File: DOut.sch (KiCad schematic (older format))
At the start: 2 parts, among them J24 Conn_02x10_Odd_Even

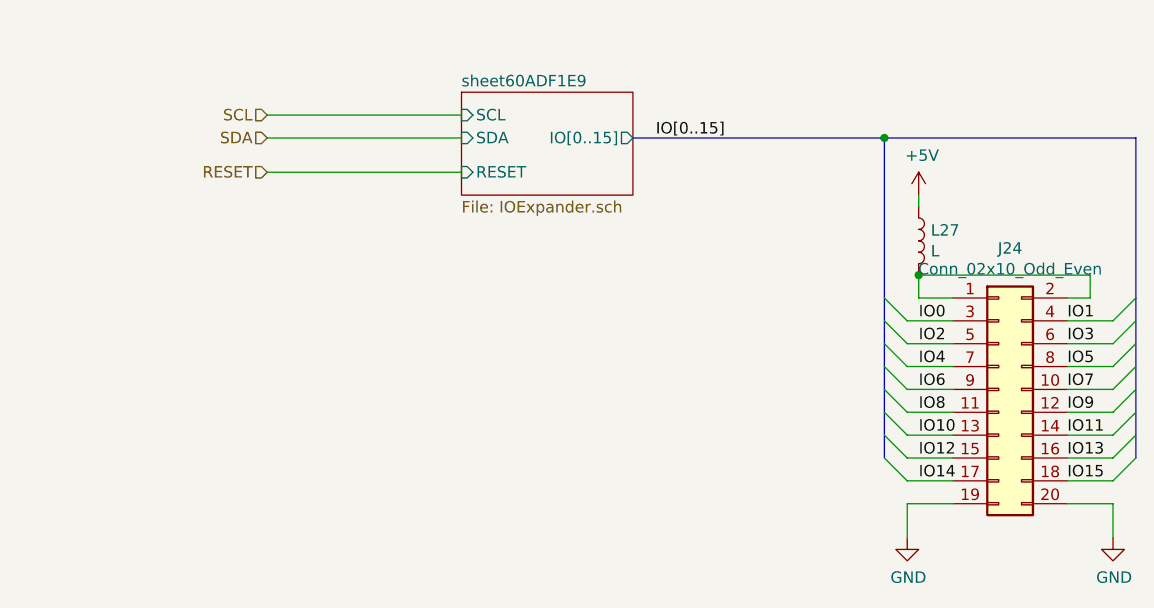
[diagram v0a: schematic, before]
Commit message: ready for jlc
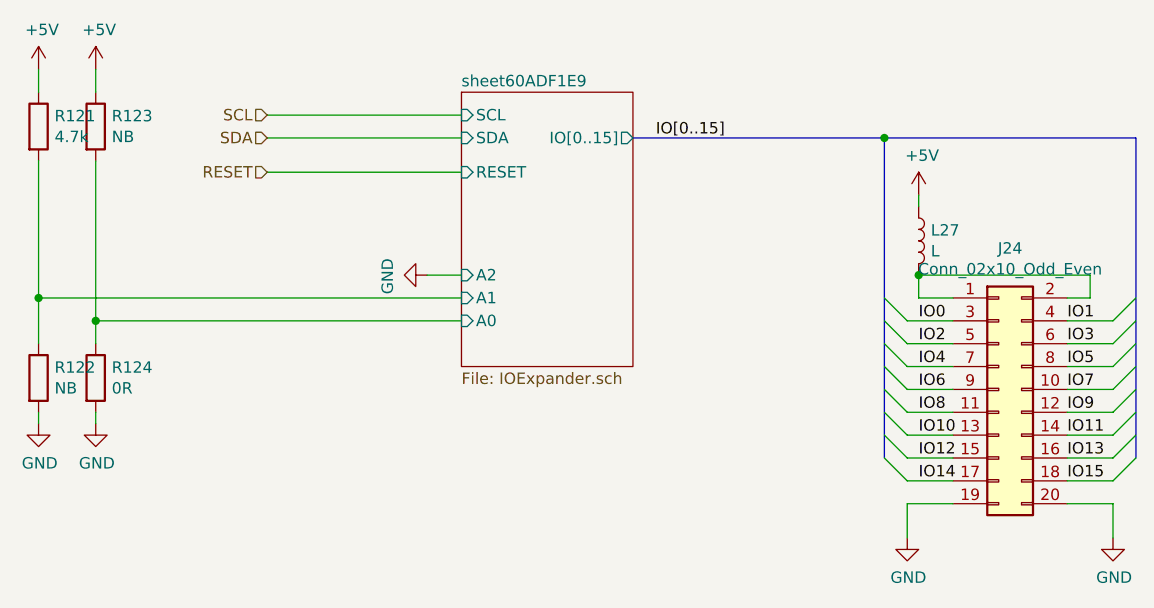
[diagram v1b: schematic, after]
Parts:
- added R121: 4.7k, Resistor_SMD:R_0603_1608Metric, symbol AR2ISS:R
- added R122, R123: NB, Resistor_SMD:R_0603_1608Metric, symbol AR2ISS:R
- added R124: 0R, Resistor_SMD:R_0603_1608Metric, symbol AR2ISS:R
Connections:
- net +5V: now also R121.1, R123.1
- net GND: now also R122.2, R124.2
- new net sheet60ADF1E9/A0: R123.2, R124.1
- new net sheet60ADF1E9/A1: R121.2, R122.1
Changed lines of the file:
@@
 $Descr A4 11693 8268
 encoding utf-8
-Sheet 12 22
+Sheet 11 22
 Title ""
 Date ""
@@
 $EndDescr
 $Sheet
-S 4650 2300 750  450
+S 4650 2300 750  1200
 U 60ADF1EF
 F0 "sheet60ADF1E9" 50
@@
 F4 "RESET" I L 4650 2650 50
 F5 "IO[0..15]" O R 5400 2500 50
+F6 "A0" I L 4650 3300 50
+F7 "A1" I L 4650 3200 50
+F8 "A2" I L 4650 3100 50
 $EndSheet
 Text HLabel 3800 2400 0    50   Input ~ 0
@@
 Text Label 7300 4000 0    50   ~ 0
 IO15
+$Comp
+L AR2ISS:R R?
+U 1 1 60A7591A
+P 3050 3550
+AR Path="/60679D69/60A7591A" Ref="R?"  Part="1"
+AR Path="/607267A8/60A7591A" Ref="R?"  Part="1"
+AR Path="/60A2B663/60A7591A" Ref="R?"  Part="1"
+AR Path="/60A2BC9C/60A7591A" Ref="R?"  Part="1"
+AR Path="/60ADDFFD/60A7591A" Ref="R?"  Part="1"
+AR Path="/60ADEB0F/60ADF1EF/60A7591A" Ref="R?"  Part="1"
+AR Path="/60A7591A" Ref="R?"  Part="1"
+AR Path="/60ADEB0F/60A7591A" Ref="R124"  Part="1"
+F 0 "R124" H 3120 3596 50  0000 L CNN
+F 1 "0R" H 3120 3505 50  0000 L CNN
+F 2 "Resistor_SMD:R_0603_1608Metric" V 2980 3550 50  0001 C CNN
+F 3 "~" H 3050 3550 50  0001 C CNN
+	1    3050 3550
+	1    0    0    -1
+$EndComp
+$Comp
+L power:GND #PWR?
+U 1 1 60A75920
+P 3050 3750
+AR Path="/607267A8/60A75920" Ref="#PWR?"  Part="1"
+AR Path="/60679D69/60A75920" Ref="#PWR?"  Part="1"
+AR Path="/60A2B663/60A75920" Ref="#PWR?"  Part="1"
+AR Path="/60A2BC9C/60A75920" Ref="#PWR?"  Part="1"
+AR Path="/60ADDFFD/60A75920" Ref="#PWR?"  Part="1"
+AR Path="/60ADEB0F/60ADF1EF/60A75920" Ref="#PWR?"  Part="1"
+AR Path="/60A75920" Ref="#PWR?"  Part="1"
+AR Path="/60ADEB0F/60A75920" Ref="#PWR0176"  Part="1"
+F 0 "#PWR0176" H 3050 3500 50  0001 C CNN
+F 1 "GND" H 3055 3577 50  0000 C CNN
+F 2 "" H 3050 3750 50  0001 C CNN
+F 3 "" H 3050 3750 50  0001 C CNN
+	1    3050 3750
+	1    0    0    -1
+$EndComp
+Wire Wire Line
+	3050 3700 3050 3750
+$Comp
+L AR2ISS:R R?
+U 1 1 60A75927
+P 2800 3550
+AR Path="/60679D69/60A75927" Ref="R?"  Part="1"
+AR Path="/607267A8/60A75927" Ref="R?"  Part="1"
+AR Path="/60A2B663/60A75927" Ref="R?"  Part="1"
+AR Path="/60A2BC9C/60A75927" Ref="R?"  Part="1"
+AR Path="/60ADDFFD/60A75927" Ref="R?"  Part="1"
+AR Path="/60ADEB0F/60ADF1EF/60A75927" Ref="R?"  Part="1"
+AR Path="/60A75927" Ref="R?"  Part="1"
+AR Path="/60ADEB0F/60A75927" Ref="R122"  Part="1"
+F 0 "R122" H 2870 3596 50  0000 L CNN
+F 1 "NB" H 2870 3505 50  0000 L CNN
+F 2 "Resistor_SMD:R_0603_1608Metric" V 2730 3550 50  0001 C CNN
+F 3 "~" H 2800 3550 50  0001 C CNN
+	1    2800 3550
+	1    0    0    -1
+$EndComp
+$Comp
+L power:GND #PWR?
+U 1 1 60A7592D
+P 2800 3750
+AR Path="/607267A8/60A7592D" Ref="#PWR?"  Part="1"
+AR Path="/60679D69/60A7592D" Ref="#PWR?"  Part="1"
+AR Path="/60A2B663/60A7592D" Ref="#PWR?"  Part="1"
+AR Path="/60A2BC9C/60A7592D" Ref="#PWR?"  Part="1"
+AR Path="/60ADDFFD/60A7592D" Ref="#PWR?"  Part="1"
+AR Path="/60ADEB0F/60ADF1EF/60A7592D" Ref="#PWR?"  Part="1"
+AR Path="/60A7592D" Ref="#PWR?"  Part="1"
+AR Path="/60ADEB0F/60A7592D" Ref="#PWR0177"  Part="1"
+F 0 "#PWR0177" H 2800 3500 50  0001 C CNN
+F 1 "GND" H 2805 3577 50  0000 C CNN
+F 2 "" H 2800 3750 50  0001 C CNN
+F 3 "" H 2800 3750 50  0001 C CNN
+	1    2800 3750
+	1    0    0    -1
+$EndComp
+Wire Wire Line
+	2800 3700 2800 3750
+$Comp
+L power:+5V #PWR?
+U 1 1 60A75934
+P 3050 2200
+AR Path="/607267A8/60A75934" Ref="#PWR?"  Part="1"
+AR Path="/60679D69/60A75934" Ref="#PWR?"  Part="1"
+AR Path="/60A2B663/60A75934" Ref="#PWR?"  Part="1"
+AR Path="/60A2BC9C/60A75934" Ref="#PWR?"  Part="1"
+AR Path="/60ADDFFD/60A75934" Ref="#PWR?"  Part="1"
+AR Path="/60ADEB0F/60ADF1EF/60A75934" Ref="#PWR?"  Part="1"
+AR Path="/60A75934" Ref="#PWR?"  Part="1"
+AR Path="/60ADEB0F/60A75934" Ref="#PWR0178"  Part="1"
+F 0 "#PWR0178" H 3050 2050 50  0001 C CNN
+F 1 "+5V" H 3065 2373 50  0000 C CNN
+F 2 "" H 3050 2200 50  0001 C CNN
+F 3 "" H 3050 2200 50  0001 C CNN
+	1    3050 2200
+	1    0    0    -1
+$EndComp
+$Comp
+L power:+5V #PWR?
+U 1 1 60A7593A
+P 2800 2200
+AR Path="/607267A8/60A7593A" Ref="#PWR?"  Part="1"
+AR Path="/60679D69/60A7593A" Ref="#PWR?"  Part="1"
+AR Path="/60A2B663/60A7593A" Ref="#PWR?"  Part="1"
+AR Path="/60A2BC9C/60A7593A" Ref="#PWR?"  Part="1"
+AR Path="/60ADDFFD/60A7593A" Ref="#PWR?"  Part="1"
+AR Path="/60ADEB0F/60ADF1EF/60A7593A" Ref="#PWR?"  Part="1"
+AR Path="/60A7593A" Ref="#PWR?"  Part="1"
+AR Path="/60ADEB0F/60A7593A" Ref="#PWR0213"  Part="1"
+F 0 "#PWR0213" H 2800 2050 50  0001 C CNN
+F 1 "+5V" H 2815 2373 50  0000 C CNN
+F 2 "" H 2800 2200 50  0001 C CNN
+F 3 "" H 2800 2200 50  0001 C CNN
+	1    2800 2200
+	1    0    0    -1
+$EndComp
+Wire Wire Line
+	2800 3200 2800 3400
+Connection ~ 2800 3200
+Wire Wire Line
+	3050 3400 3050 3300
+Connection ~ 3050 3300
+Wire Wire Line
+	2800 3200 4650 3200
+Wire Wire Line
+	3050 3300 4650 3300
+$Comp
+L AR2ISS:R R?
+U 1 1 60A75947
+P 2800 2450
+AR Path="/60679D69/60A75947" Ref="R?"  Part="1"
+AR Path="/607267A8/60A75947" Ref="R?"  Part="1"
+AR Path="/60A2B663/60A75947" Ref="R?"  Part="1"
+AR Path="/60A2BC9C/60A75947" Ref="R?"  Part="1"
+AR Path="/60ADDFFD/60A75947" Ref="R?"  Part="1"
+AR Path="/60ADEB0F/60ADF1EF/60A75947" Ref="R?"  Part="1"
+AR Path="/60A75947" Ref="R?"  Part="1"
+AR Path="/60ADEB0F/60A75947" Ref="R121"  Part="1"
+F 0 "R121" H 2870 2496 50  0000 L CNN
+F 1 "4.7k" H 2870 2405 50  0000 L CNN
+F 2 "Resistor_SMD:R_0603_1608Metric" V 2730 2450 50  0001 C CNN
+F 3 "~" H 2800 2450 50  0001 C CNN
+	1    2800 2450
+	1    0    0    -1
+$EndComp
+$Comp
+L AR2ISS:R R?
+U 1 1 60A7594D
+P 3050 2450
+AR Path="/60679D69/60A7594D" Ref="R?"  Part="1"
+AR Path="/607267A8/60A7594D" Ref="R?"  Part="1"
+AR Path="/60A2B663/60A7594D" Ref="R?"  Part="1"
+AR Path="/60A2BC9C/60A7594D" Ref="R?"  Part="1"
+AR Path="/60ADDFFD/60A7594D" Ref="R?"  Part="1"
+AR Path="/60ADEB0F/60ADF1EF/60A7594D" Ref="R?"  Part="1"
+AR Path="/60A7594D" Ref="R?"  Part="1"
+AR Path="/60ADEB0F/60A7594D" Ref="R123"  Part="1"
+F 0 "R123" H 3120 2496 50  0000 L CNN
+F 1 "NB" H 3120 2405 50  0000 L CNN
+F 2 "Resistor_SMD:R_0603_1608Metric" V 2980 2450 50  0001 C CNN
+F 3 "~" H 3050 2450 50  0001 C CNN
+	1    3050 2450
+	1    0    0    -1
+$EndComp
+Wire Wire Line
+	3050 2600 3050 3300
+Wire Wire Line
+	2800 2600 2800 3200
+Wire Wire Line
+	2800 2300 2800 2200
+Wire Wire Line
+	3050 2200 3050 2300
+$Comp
+L power:GND #PWR?
+U 1 1 60A7B8D9
+P 4500 3100
+AR Path="/607267A8/60A7B8D9" Ref="#PWR?"  Part="1"
+AR Path="/60679D69/60A7B8D9" Ref="#PWR?"  Part="1"
+AR Path="/60A2B663/60A7B8D9" Ref="#PWR?"  Part="1"
+AR Path="/60A2BC9C/60A7B8D9" Ref="#PWR?"  Part="1"
+AR Path="/60ADDFFD/60A7B8D9" Ref="#PWR?"  Part="1"
+AR Path="/60ADEB0F/60ADF1EF/60A7B8D9" Ref="#PWR?"  Part="1"
+AR Path="/60A7B8D9" Ref="#PWR?"  Part="1"
+AR Path="/60ADEB0F/60A7B8D9" Ref="#PWR0216"  Part="1"
+F 0 "#PWR0216" H 4500 2850 50  0001 C CNN
+F 1 "GND" H 4505 2927 50  0000 C CNN
+F 2 "" H 4500 3100 50  0001 C CNN
+F 3 "" H 4500 3100 50  0001 C CNN
+	1    4500 3100
+	0    1    1    0
+$EndComp
+Wire Wire Line
+	4500 3100 4650 3100
 Wire Bus Line
 	6500 2500 6500 3900
